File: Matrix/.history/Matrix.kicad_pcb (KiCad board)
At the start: 2 copper layers, 150 x 150 mm, 173 parts, among them J1 Conn_01x08, J2 USB_C_Receptacle_USB2.0_16P, Q1 2N2219, Q10 2N2219, Q11 2N2219, Q12 2N2219, Q13 2N2219, Q14 2N2219, Q15 2N2219, Q16 2N2219, Q2 2N2219, Q3 2N2219, Q4 2N2219, Q5 2N2219, Q6 2N2219, Q7 2N2219, Q8 2N2219, Q9 2N2219, SW1 SW_Push, SW2 SW_Push, U1 74HC138, U10 ESP32-S3, U11 AP2112K-3.3, U12 ER_OLEDM0.91_1x-I2C, U13 W25Q32JVSS, U2 74HC574N, U3 74HC574N, U4 74HC574N, U5 74HC574N, U6 74HC574N, U7 74HC574N, U8 74HC574N, U9 74HC574N, Y1 40MHz (+-10ppm)

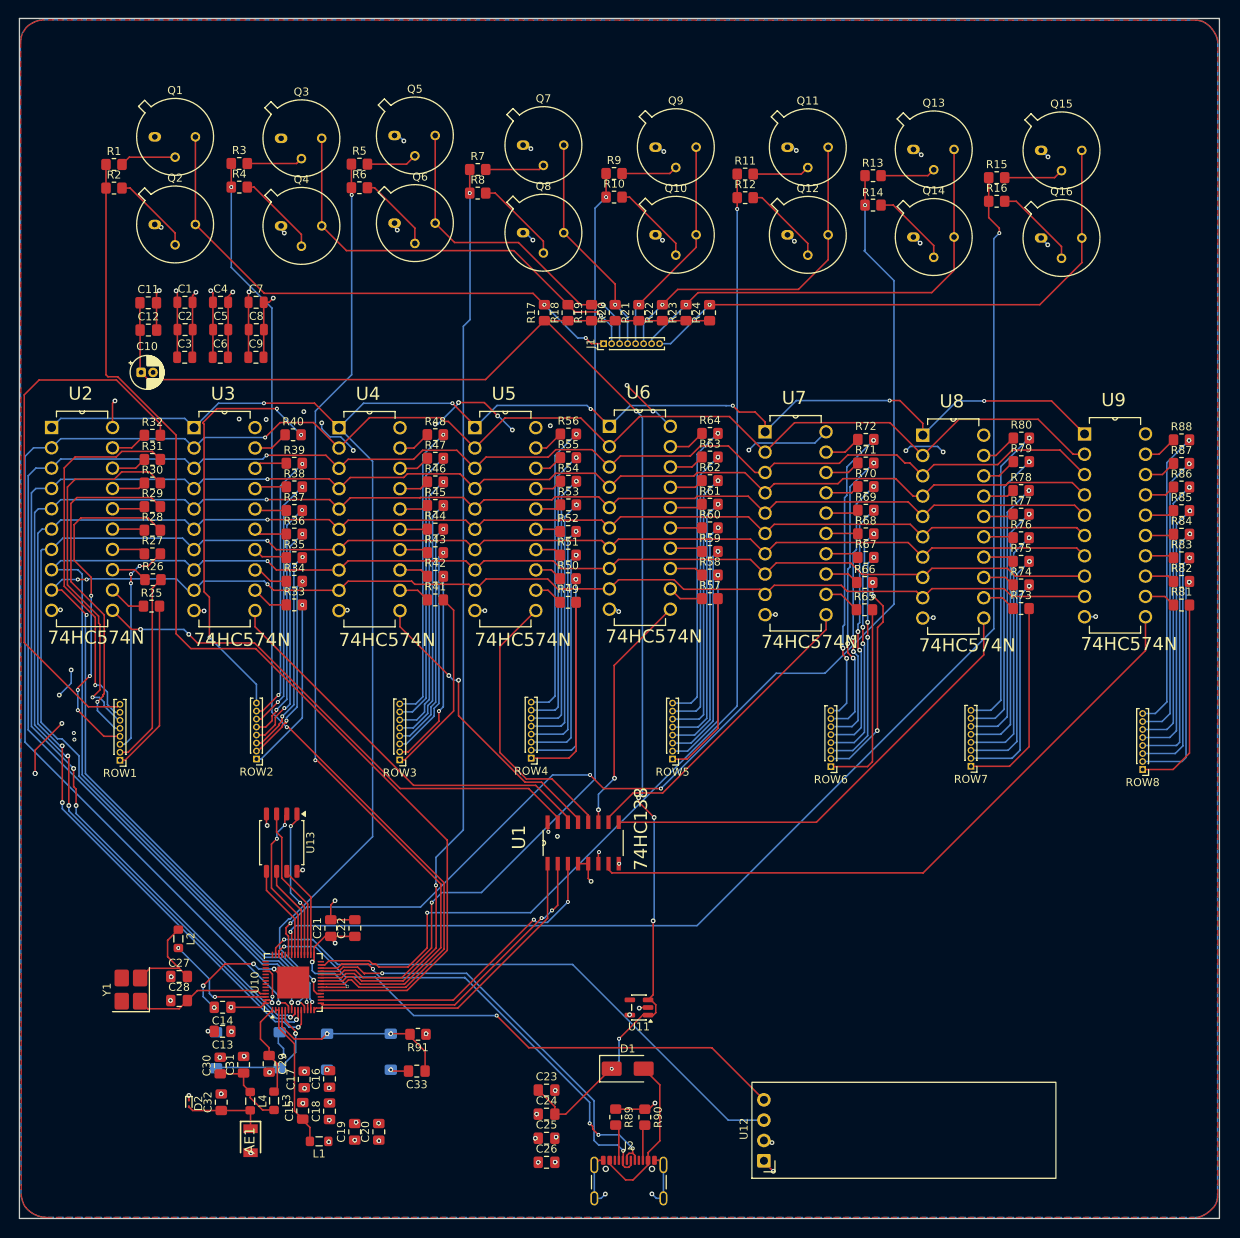
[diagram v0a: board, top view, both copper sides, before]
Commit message: Update Matrix.kicad_pcb
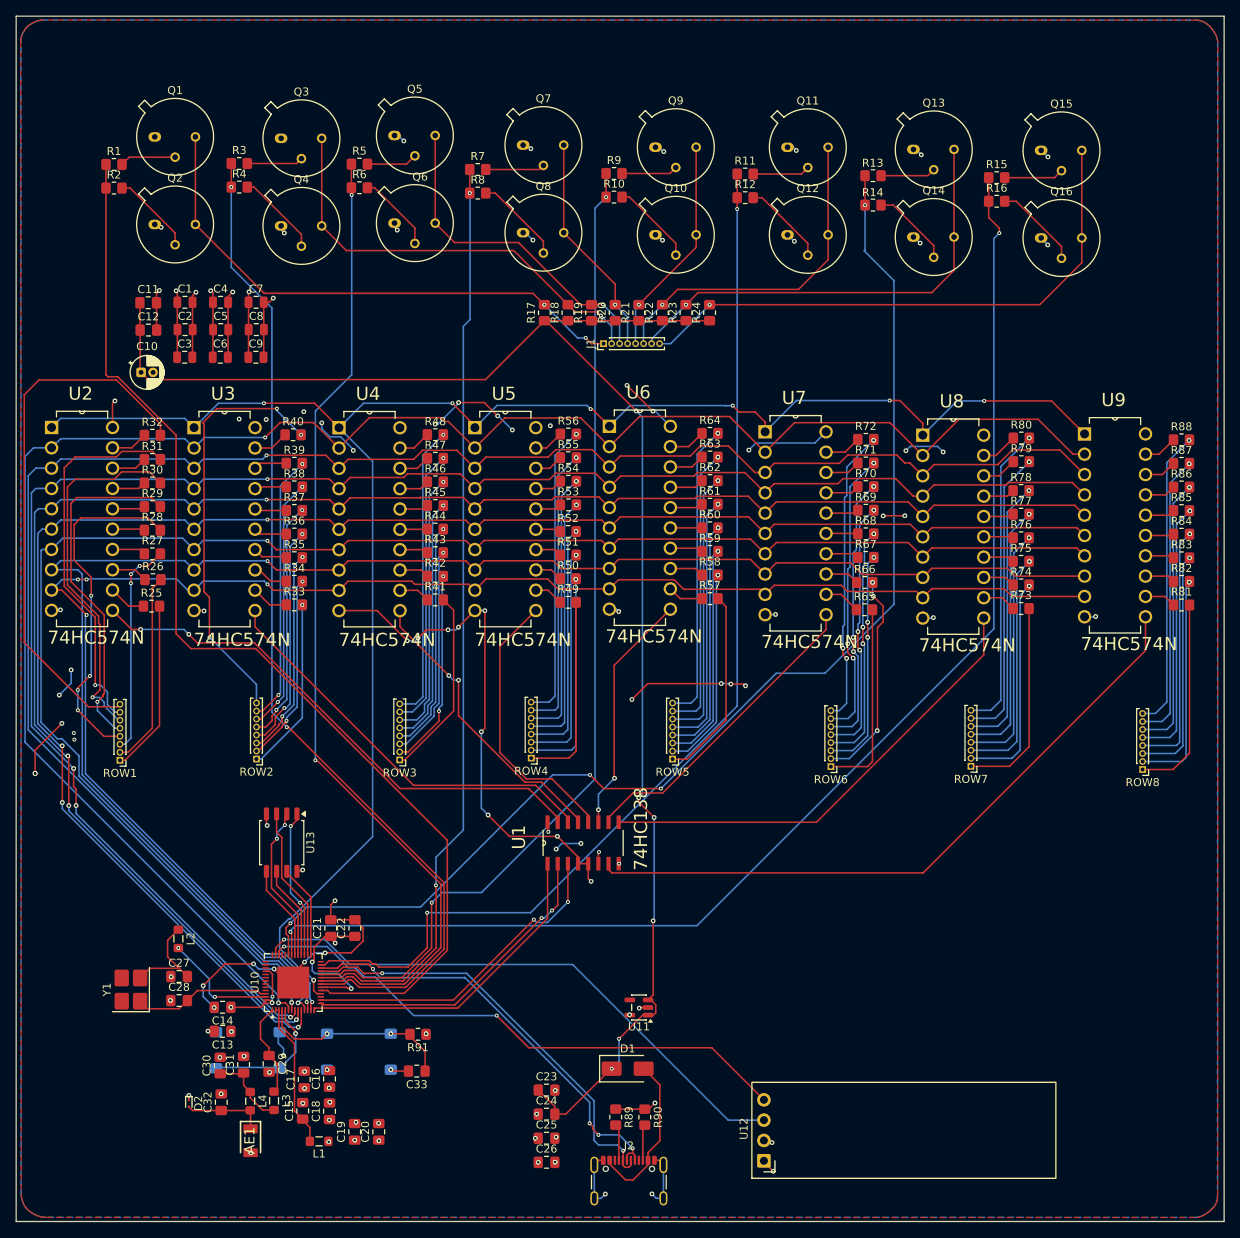
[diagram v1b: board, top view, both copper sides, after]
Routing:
- net GND: track 123.6 -> 215.5 mm, vias 65 -> 78
- net +3.3V: track 108.5 -> 113.1 mm, vias 43 -> 45
- net Net-(ROW5-Pin_1): track 23.5 -> 24.3 mm
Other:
- board size 150 x 150 mm -> 151 x 150.7 mm
